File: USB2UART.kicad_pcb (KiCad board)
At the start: 2 copper layers, 43.9 x 34.3 mm, 33 parts, among them J1 Conn_01x04, J2 Conn_01x03, J3 Conn_01x03, J4 Conn_01x04, J5 Conn_01x04, Q1 S8050, U3 HX9193, U6 SL2.1S, U7 CH340E, U8 CH340E, Y1 12M

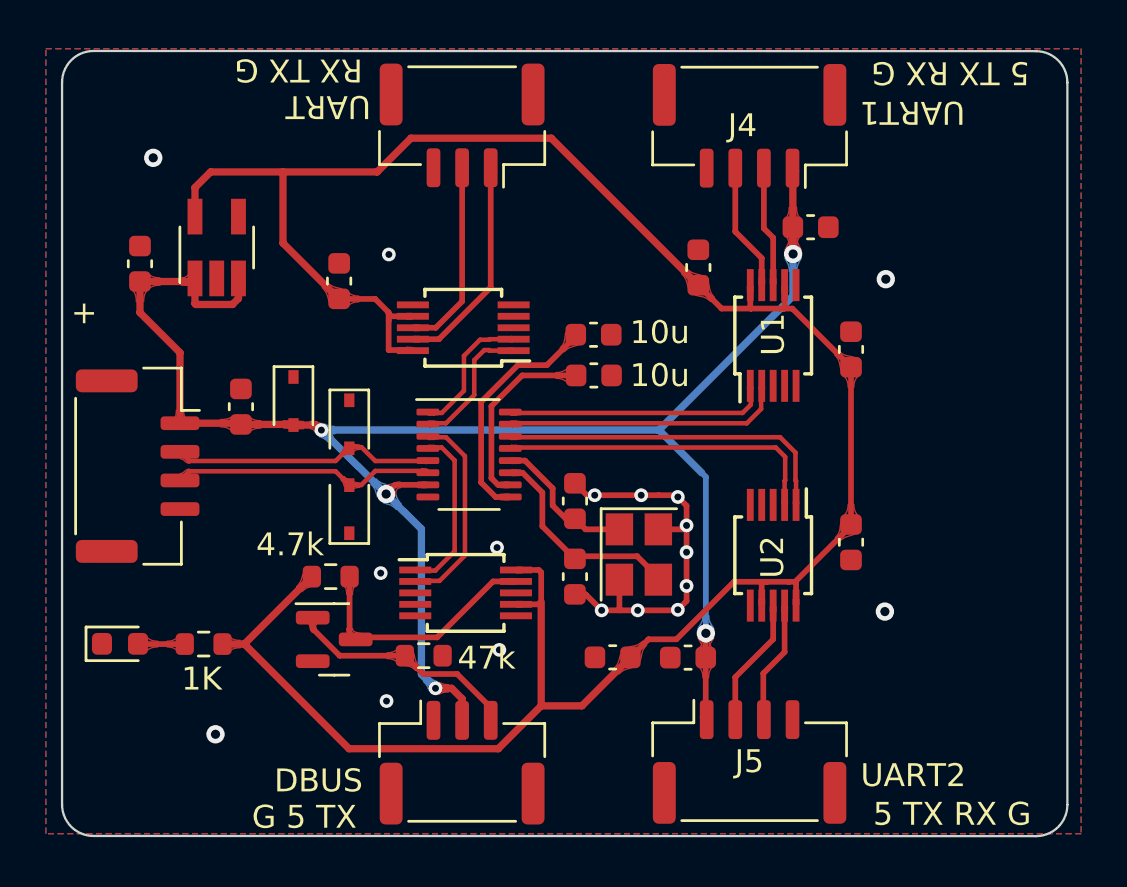
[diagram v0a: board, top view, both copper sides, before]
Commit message: iterative optimization
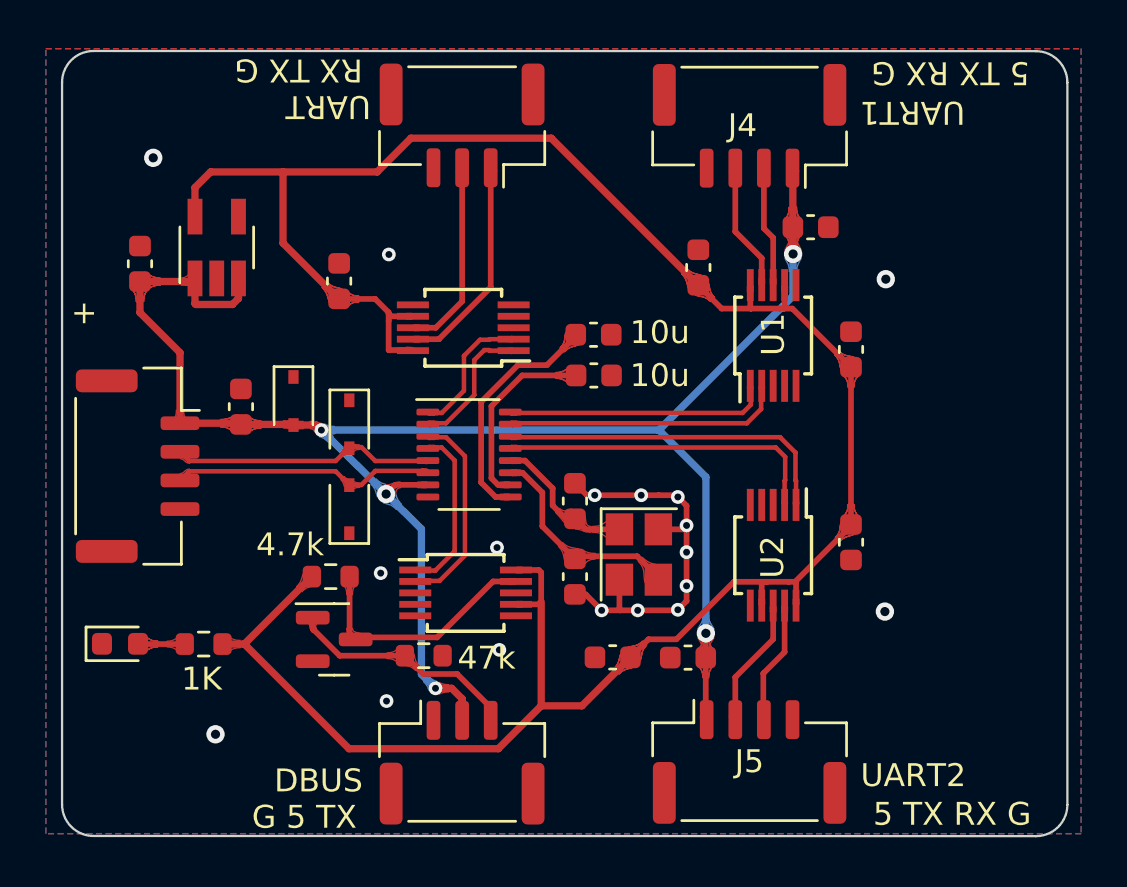
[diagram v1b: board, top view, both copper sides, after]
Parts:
- C1, C2: value ~ -> 100n
- U1, U2: value ~ -> CH340E
